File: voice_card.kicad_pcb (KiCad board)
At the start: 2 copper layers, 119.3 x 38 mm, 207 parts, among them J1 PCI_11_49, Q1 MMBF4391LT1G, Q10 DMMT3906, Q11 BC857BS, Q2 2N3904, Q3 BCM847, Q4 DMMT3904, Q5 DMMT3906, Q6 MMBF4391LT1G, Q7 BCM847, Q8 2N3904, Q9 DMMT3904, U1 TL074-, U10 TL072-, U11 TL074-, U12 NE555, U13 LM311M, U14 CD4052, U15 TL072-, U16 TL072-, U17 LM13700, U18 LM13700, U19 LM13700, U2 TL074-, U20 TL072-, U3 NE555, U4 LF351, U5 TL072-, U6 LM311M, U7 CD4052, U8 TL074-, U9 LF351

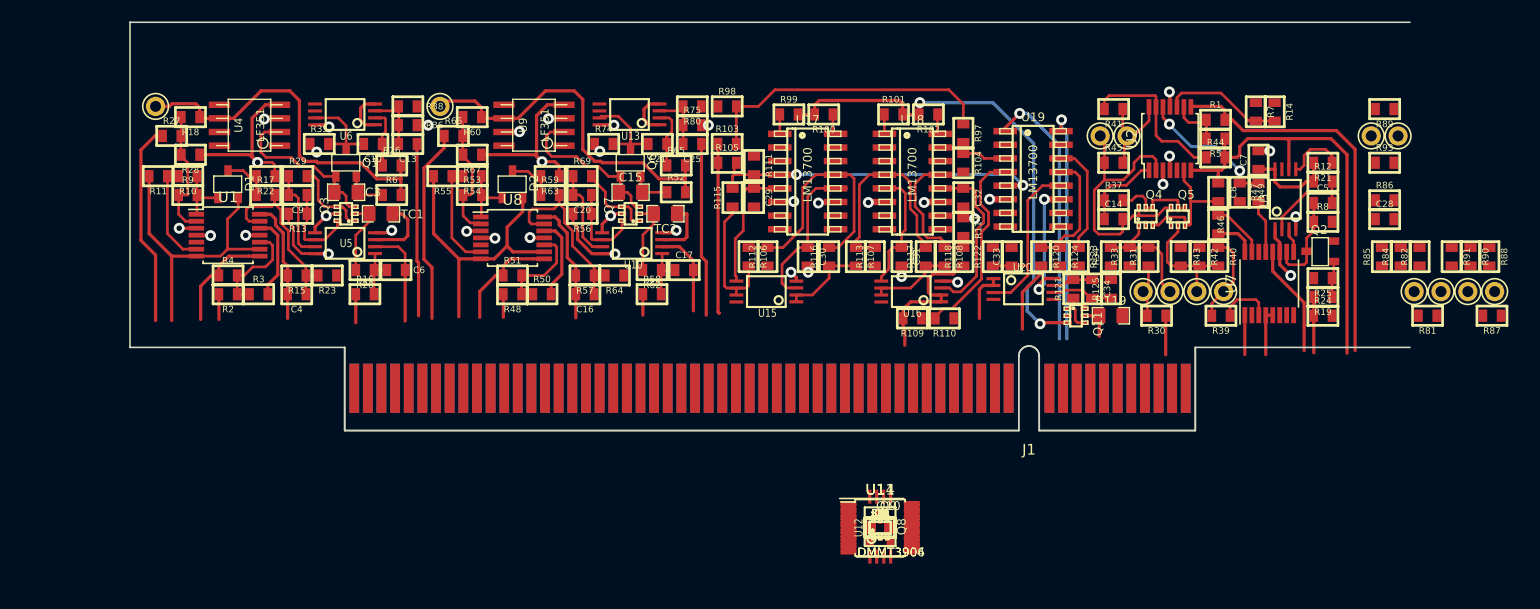
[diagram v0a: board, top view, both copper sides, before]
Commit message: EG2 placed and routed
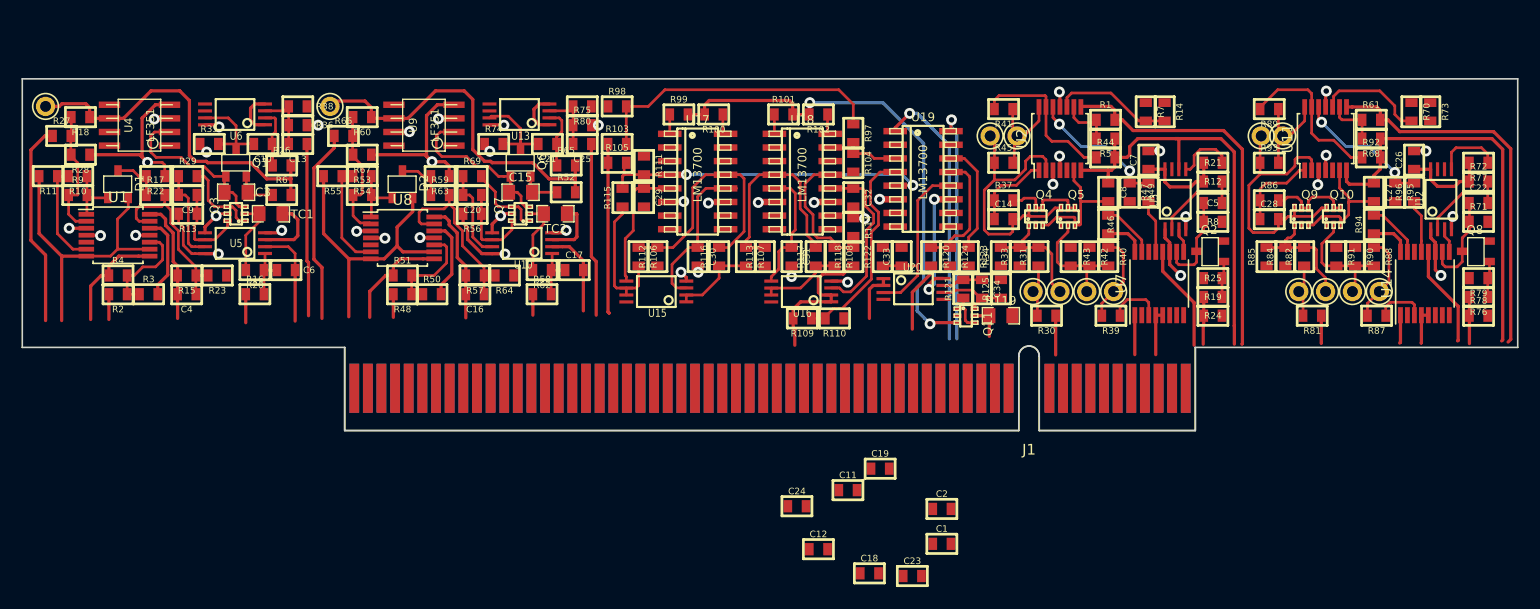
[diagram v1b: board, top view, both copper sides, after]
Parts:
- moved R77 65.3 mm to (204.2, 71.0), turned to 180 degrees
- moved R72 64.4 mm to (204.2, 72.8)
- moved R73 64.3 mm to (199.8, 66.2), turned to 270 degrees
- moved C22 63.4 mm to (204.2, 74.8)
- moved R70 62.9 mm to (198.0, 66.2), turned to 270 degrees
- moved R71 62.6 mm to (204.2, 76.5)
- moved Q8 61.2 mm to (204.0, 79.2), turned to 90 degrees
- moved U12 60.5 mm to (200.8, 74.5)
- moved R79 60.4 mm to (204.2, 81.8), turned to 180 degrees
- moved C26 60.4 mm to (198.2, 70.8), turned to 90 degrees
- moved R76 59.8 mm to (204.2, 83.5), turned to 180 degrees
- moved R61 59.5 mm to (194.2, 67.0)
- moved R78 59.1 mm to (204.2, 85.2)
- moved R96 58.8 mm to (198.2, 73.8), turned to 90 degrees
- moved R68 58.4 mm to (194.2, 68.8), turned to 180 degrees
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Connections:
- Q10 pad 1: Net-(Q10-Pad1) -> GND
- Q10 pad 2: GND -> Net-(Q10-Pad2)
- Q10 pad 3: Net-(C28-Pad2) -> Net-(C27-Pad2)
- Q10 pad 6: Net-(C27-Pad2) -> Net-(C28-Pad2)
- R88 pad 2: Net-(Q10-Pad1) -> Net-(Q10-Pad2)
- R90 pad 2: Net-(Q10-Pad1) -> Net-(Q10-Pad2)
- R91 pad 2: Net-(Q10-Pad1) -> Net-(Q10-Pad2)
- TP12 pad 1: Net-(Q10-Pad1) -> Net-(Q10-Pad2)
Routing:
- net EG2_ENV_OUT: track 0.00 -> 37.8 mm
- net EG2_INV_OUT: track 0.00 -> 35.5 mm
- net Net-(C28-Pad2): track 0.00 -> 25.7 mm
- net Net-(R89-Pad2): track 0.00 -> 15.1 mm
- net +12V: track 52.0 -> 66.8 mm, vias 15 -> 17
- net Net-(R95-Pad1): track 0.00 -> 13.1 mm, vias 0 -> 2
- net Net-(C27-Pad2): track 0.00 -> 12.2 mm
- net Net-(Q9-Pad1): track 0.00 -> 11.6 mm
- net Net-(Q10-Pad2): track 0.00 -> 11.4 mm
- net Net-(R70-Pad2): track 0.00 -> 10.1 mm
- net EG2_SUSTAIN_CV: track 0.00 -> 9.47 mm
- net Net-(R89-Pad1): track 0.00 -> 9.26 mm
- net Net-(C22-Pad1): track 0.00 -> 9.04 mm
- net Net-(C22-Pad2): track 0.00 -> 8.69 mm
- net Net-(Q10-Pad4): track 0.00 -> 8.28 mm
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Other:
- board size 119.3 x 38 mm -> 139.3 x 32.8 mm
